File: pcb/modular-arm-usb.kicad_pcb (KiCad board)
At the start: 2 copper layers, 50 x 22 mm, 30 parts, among them CON1 SWD, IC1 LPC11U14FBD48, P1 USB, P2 LED, P3 BATT, P4 GPIO, P5 gnd, P6 GPIO2, SW1 SW_SPDT, SW2 SW_PUSH_ALT, U2 MCP1700T, U3 nRF24L01+, X1 16M xtal

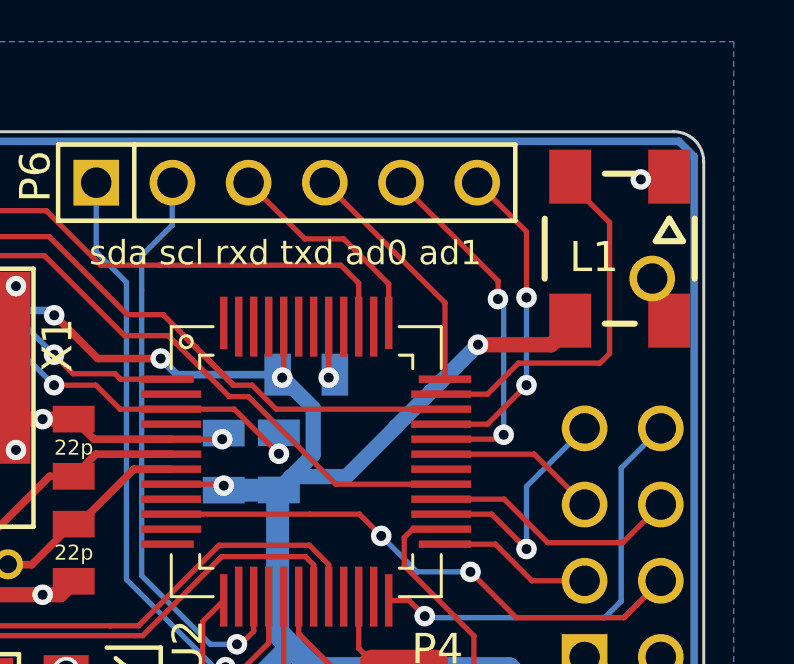
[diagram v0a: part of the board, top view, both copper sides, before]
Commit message: gerbers for oshpark order
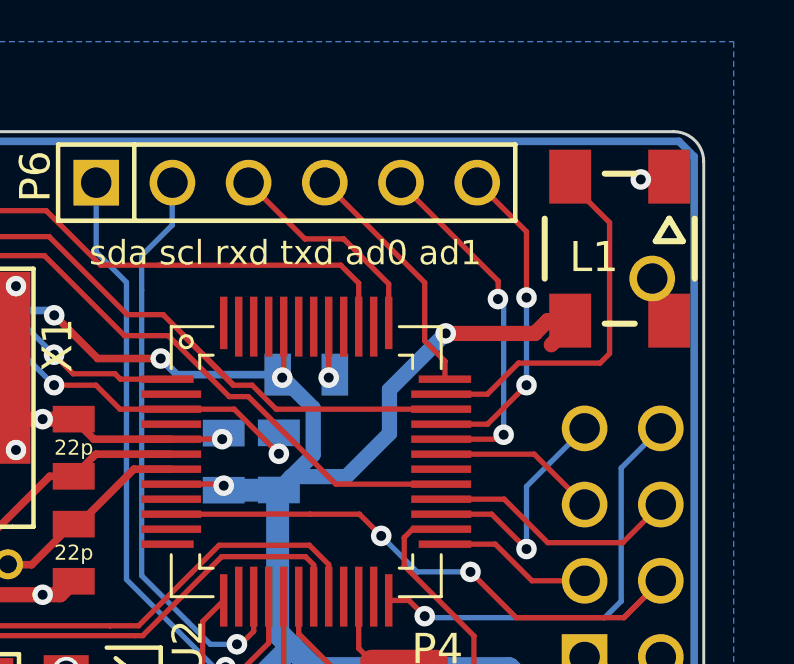
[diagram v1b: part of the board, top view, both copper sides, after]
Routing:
- net 3V3: track 103.1 -> 104.9 mm
